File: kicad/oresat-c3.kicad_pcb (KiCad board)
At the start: 4 copper layers, 90.2 x 95.9 mm, 201 parts, among them J1 Conn_02x26_Odd_Even, J2 Conn_02x26_Odd_Even, J4 Conn_01x05, J5 DM3BT-DSF-PEJS, J6 Conn_01x02, J7 2-1734592-0, Q1 NTR4101P, Q6 MMBT2907, U1 OSD3358-512M-ISM, U10 SN74AUC1G07DCKR, U11 RCLAMP0504FB, U12 RCLAMP0504FB, U14 TLVH431, U2 MR20H40CDF, U24 RV-3028-C7, U30 FM24CL64B-DGTR, U37 LTC4300A-1, U39 TCAN330, U8 TCAN330, U9 EMMC+RESET+5.1-COMPATIBLE-BA, Y1 ECS-240-12-30BQ-AEN-TR, Y2 ABS07-32.768KHZ-T

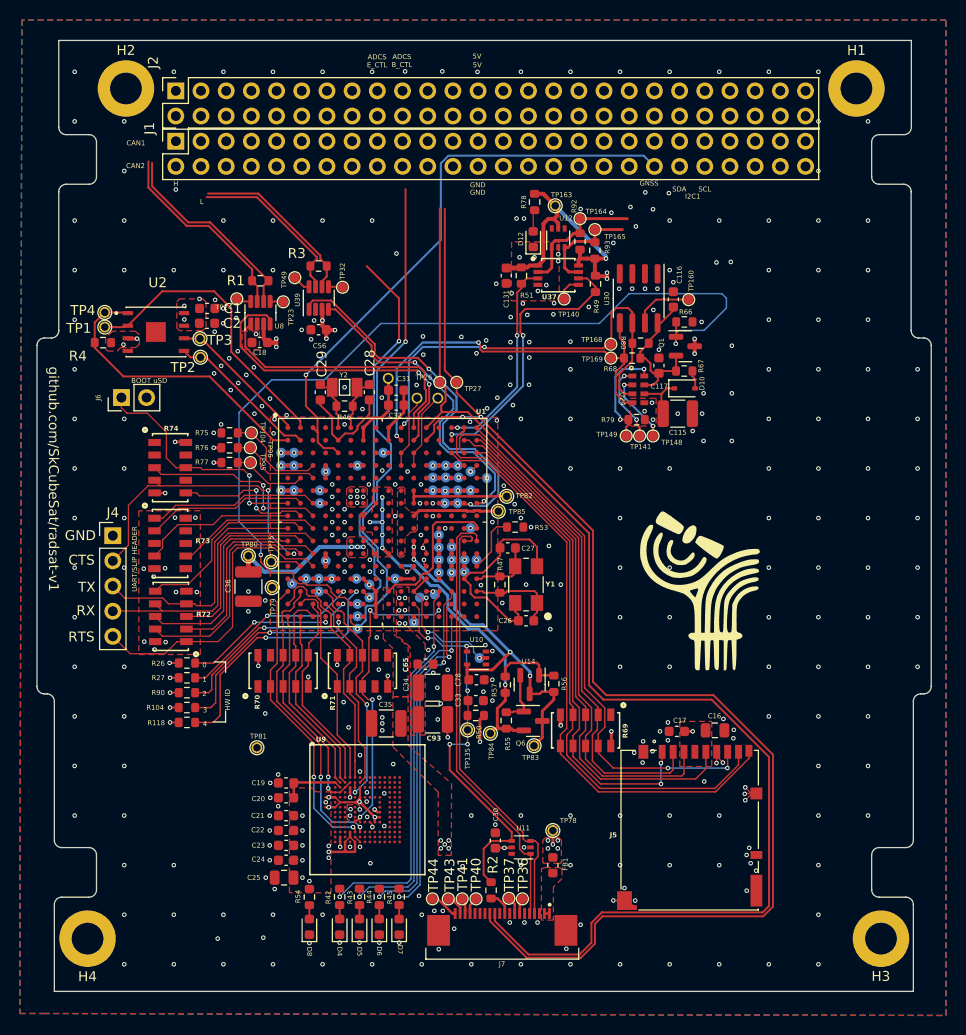
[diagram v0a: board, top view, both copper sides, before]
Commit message: Updated PCB to the new PC104 template form factor
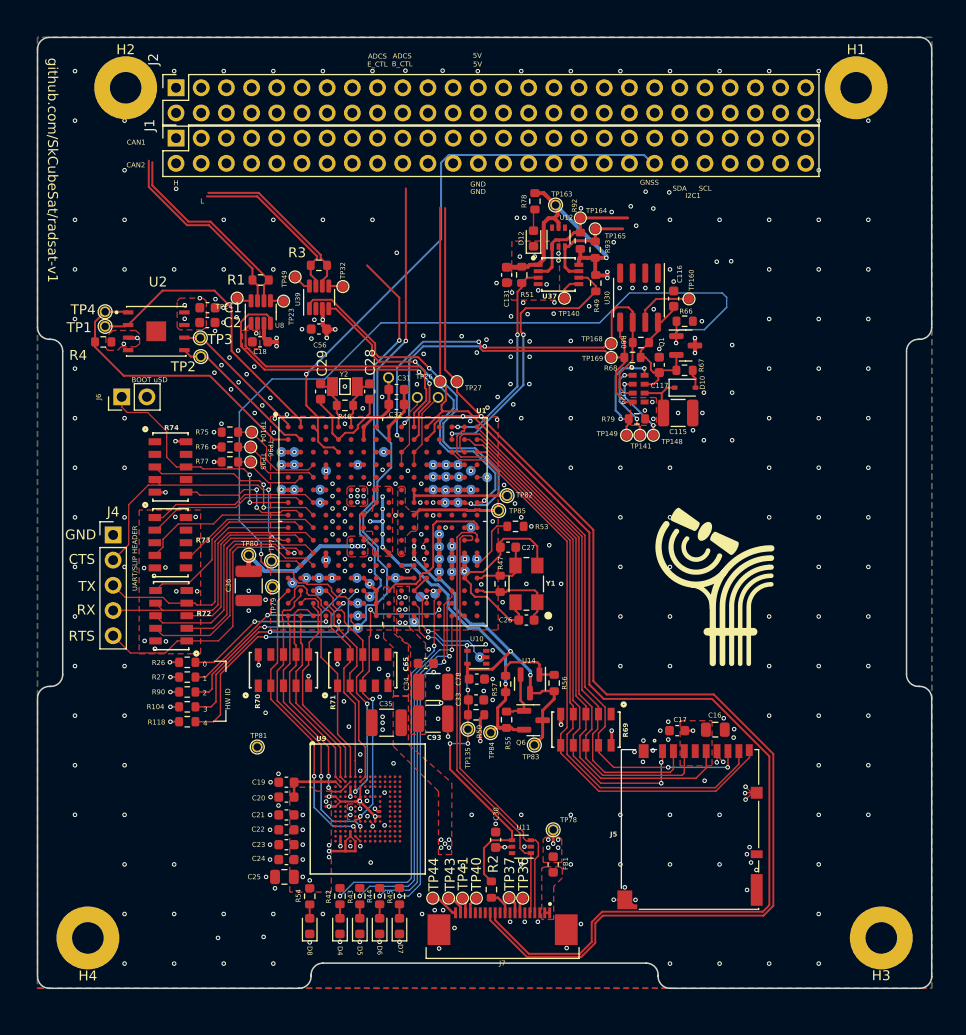
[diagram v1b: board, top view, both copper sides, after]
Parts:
- removed G***: LOGO, logos:radsatsk2-logo
- moved J2 0.31 mm to (78.1, 50.9)
- moved J1 0.31 mm to (78.1, 56.0)
- moved C2 0.08 mm to (81.3, 74.6)
- moved C56 0.08 mm to (92.5, 75.2)
- moved D12 0.08 mm to (114.2, 66.1)
- moved D4 0.08 mm to (94.6, 135.4)
- moved D5 0.08 mm to (96.6, 135.4)
- moved D6 0.08 mm to (98.6, 135.4)
- moved D7 0.08 mm to (100.6, 135.4)
- moved FB1 0.08 mm to (116.1, 129.2)
- moved J4 0.08 mm to (71.8, 96.0)
- moved Q6 0.08 mm to (114.1, 114.7)
- moved R1 0.08 mm to (86.6, 70.3)
- moved R3 0.08 mm to (92.5, 68.8)
- moved R42 0.08 mm to (94.6, 132.4)
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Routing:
- net GND: vias 387 -> 373
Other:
- outline, holes or cut-outs redrawn
